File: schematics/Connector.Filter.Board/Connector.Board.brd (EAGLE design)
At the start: 159.4 x 72.1 mm, 95 parts, among them U1 AD8244, U2 AD8244, U3 AD8244, U4 AD8244, U5 AD8244, U6 AD8244, U7 AD8244, U8 AD8244, U9 AD8244, X1 EEGCON, X2 EITCON

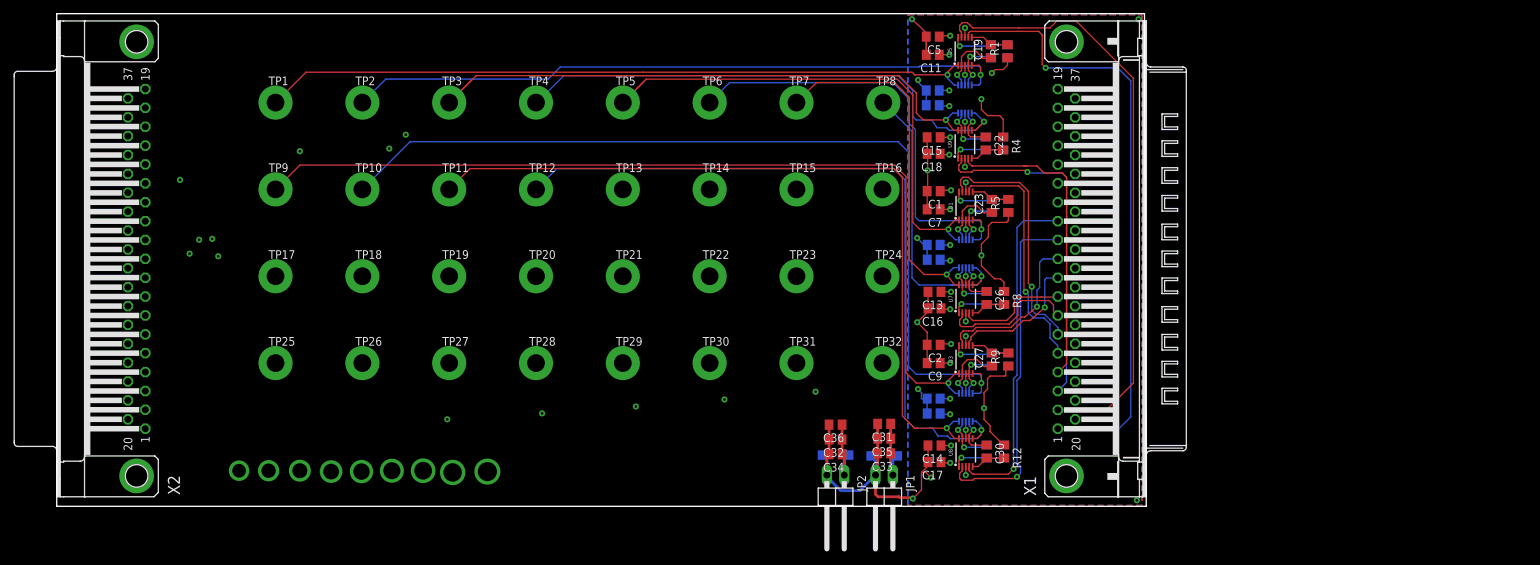
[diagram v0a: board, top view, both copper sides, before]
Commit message: Renaming Sch and Brd but not matching yet
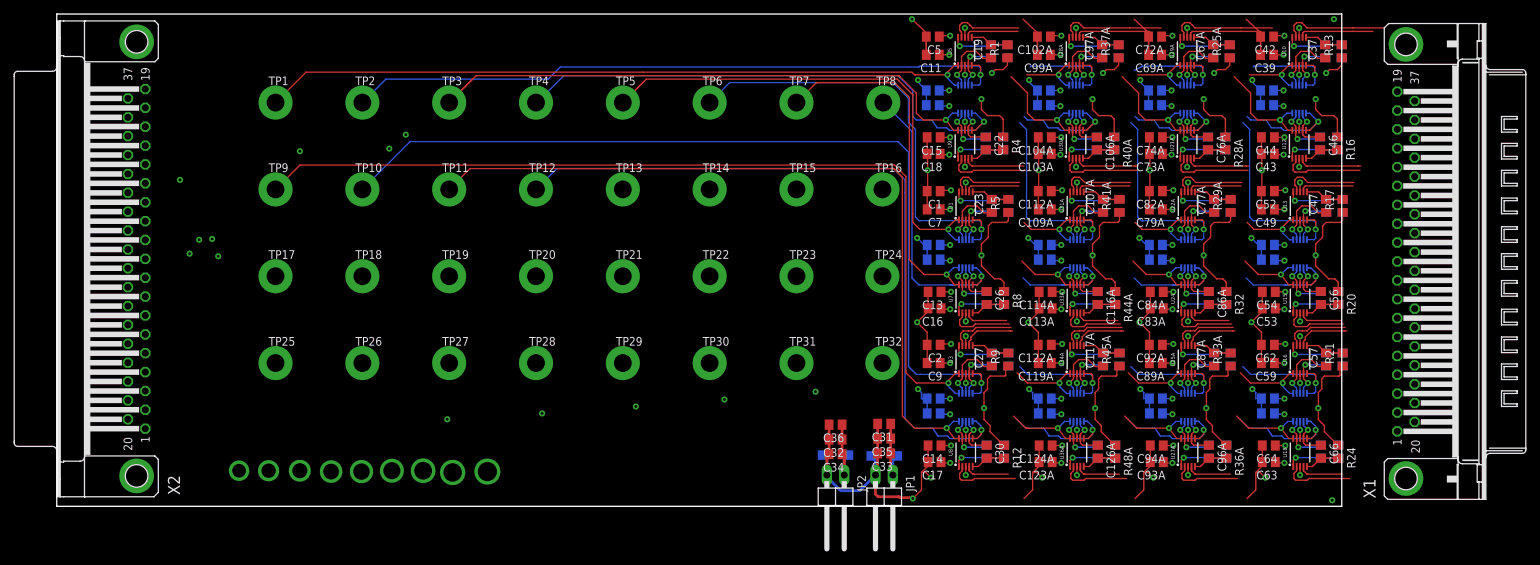
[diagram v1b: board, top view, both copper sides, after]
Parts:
- added C100A, C101A, C102A, C103A, C104A, C105A, C109A, C110A, C111A, C112A, C113A, C114A, C119A, C120A, C121A, C122A, C123A, C124A, C39, C40, C41, C42, C43, C44, C45, C49, C50, C51, C52, C53, C54, C59, C60, C61, C62, C63, C64, C69A, C70A, C71A, C72A, C73A, C74A, C75A, C79A, C80A, C81A, C82A, C83A, C84A, C89A, C90A, C91A, C92A, C93A, C94A, C99A: 0.1uF, resistor:C0805
- added C106A, C107A, C108A, C115A, C116A, C117A, C118A, C125, C126A, C37, C38, C46, C47, C48, C55, C56, C57, C58, C65, C66, C67A, C68A, C76A, C77A, C78A, C85A, C86A, C87A, C88A, C95A, C96A, C97A, C98A: (no value), resistor:C0805
- added R13, R14, R15, R16, R17, R18, R19, R20, R21, R22, R23, R24, R25A, R26A, R27A, R28A, R29A, R30A, R31, R32, R33A, R34A, R35A, R36A, R37A, R38A, R39A, R40A, R41A, R42A, R43A, R44A, R45A, R46A, R47, R48A: (no value), resistor:R0805
- added U10, U11, U12, U13, U14, U15, U16, U17, U18, U19A, U20A, U21A, U22A, U23A, U24, U25A, U26A, U27A, U28A, U29A, U30A, U31A, U32A, U33A, U34A, U35A, U36A: AD8244, AD8244:MSOP10
- moved X1 49.7 mm to (198.2, 55.2)
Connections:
- new net BUF13: C37.1, C97A.1, U10.2, U11.2, U28A.2, U29A.2
- new net BUF14: C38.1, C98A.1, U10.4, U11.4, U28A.4, U29A.4
- new net BUF15: C105A.1, C45.1, U11.9, U12.9, U29A.9, U30A.9
- new net BUF16: C106A.1, C46.1, U11.7, U12.7, U29A.7, U30A.7
- new net BUF17: C107A.1, C47.1, U13.2, U14.2, U31A.2, U32A.2
- new net BUF18: C108A.1, C48.1, U13.4, U14.4, U31A.4, U32A.4
- new net BUF19: C115A.1, C55.1, U14.9, U15.9, U32A.9, U33A.9
- new net BUF20: C116A.1, C56.1, U14.7, U15.7, U32A.7, U33A.7
- new net BUF21: C117A.1, C57.1, U16.2, U17.2, U34A.2, U35A.2
- new net BUF22: C118A.1, C58.1, U16.4, U17.4, U34A.4, U35A.4
- new net BUF23: C125.1, C65.1, U17.9, U18.9, U35A.9, U36A.9
- new net BUF24: C126A.1, C66.1, U17.7, U18.7, U35A.7, U36A.7
- new net BUF25: C67A.1, U19A.2, U20A.2
- new net BUF26: C68A.1, U19A.4, U20A.4
- new net BUF27: C75A.1, U20A.9, U21A.9
- new net BUF28: C76A.1, U20A.7, U21A.7
- new net BUF29: C77A.1, U22A.2, U23A.2
- new net BUF30: C78A.1, U22A.4, U23A.4
- new net BUF31: C85A.1, U23A.9, U24.9
- new net BUF32: C86A.1, U23A.7, U24.7
- new net BUF33: C87A.1, U25A.2, U26A.2
- new net BUF34: C88A.1, U25A.4, U26A.4
- new net BUF35: C95A.1, U26A.9, U27A.9
- new net BUF36: C96A.1, U26A.7, U27A.7
- new net FILT10_BUF1: U16.9
- new net FILT10_BUF2: U25A.9
- new net FILT10_OUT1: C58.2, R22.2, U16.10
- new net FILT10_OUT2: C88A.2, R34A.2, U25A.10
- new net FILT11_BUF1: U18.2
- new net FILT11_BUF2: U27A.2
- new net FILT11_OUT1: C65.2, R23.2, U18.1
- new net FILT11_OUT2: C95A.2, R35A.2, U27A.1
- new net FILT12_BUF1: U18.4
- new net FILT12_BUF2: U27A.4
- new net FILT12_OUT1: C66.2, R24.2, U18.5
- new net FILT12_OUT2: C96A.2, R36A.2, U27A.5
- new net FILT14_OUT: C98A.2, R38A.2, U28A.10
- new net FILT15_OUT: C105A.2, R39A.2, U30A.1
- new net FILT16_OUT: C106A.2, R40A.2, U30A.5
- new net FILT17_OUT: C107A.2, R41A.2, U31A.6
- new net FILT18_OUT: C108A.2, R42A.2, U31A.10
- new net FILT19_OUT: C115A.2, R43A.2, U33A.1
- new net FILT1_BUF1: U10.7
- new net FILT1_OUT1: C37.2, R13.2, U10.6
- new net FILT20_OUT: C116A.2, R44A.2, U33A.5
- new net FILT21_OUT: C117A.2, R45A.2, U34A.6
- new net FILT22_OUT: C118A.2, R46A.2, U34A.10
- new net FILT23_OUT: C125.2, R47.2, U36A.1
- new net FILT24_OUT: C126A.2, R48A.2, U36A.5
- new net FILT25_OUT: C67A.2, R25A.2, U19A.6
- new net FILT26_OUT: C68A.2, R26A.2, U19A.10
- new net FILT27_OUT: C75A.2, R27A.2, U21A.1
- new net FILT28_OUT: C76A.2, R28A.2, U21A.5
- new net FILT2_BUF1: U10.9
- new net FILT2_OUT1: C38.2, R14.2, U10.10
- new net FILT31_OUT: C85A.2, R31.2, U24.1
- new net FILT32_OUT: C86A.2, R32.2, U24.5
- new net FILT3_BUF1: U12.2
- new net FILT3_OUT1: C45.2, R15.2, U12.1
- new net FILT4_BUF1: U12.4
- new net FILT4_OUT1: C46.2, R16.2, U12.5
- new net FILT5_BUF1: U13.7
- new net FILT5_BUF2: U22A.7
- new net FILT5_OUT1: C47.2, R17.2, U13.6
- new net FILT5_OUT2: C77A.2, R29A.2, U22A.6
- new net FILT6_BUF1: U13.9
- new net FILT6_BUF2: U22A.9
- new net FILT6_OUT1: C48.2, R18.2, U13.10
- new net FILT6_OUT2: C78A.2, R30A.2, U22A.10
- new net FILT7_BUF1: U15.2
- new net FILT7_OUT1: C55.2, R19.2, U15.1
- new net FILT8_BUF1: U15.4
- new net FILT8_OUT1: C56.2, R20.2, U15.5
- new net FILT9_BUF1: U16.7
- new net FILT9_BUF2: U25A.7
- new net FILT9_OUT1: C57.2, R21.2, U16.6
- new net FILT9_OUT2: C87A.2, R33A.2, U25A.6
- new net PIN33: U10.1, U11.1
- new net PIN34: U10.5, U11.5
- new net PIN35: U11.10, U12.10
- new net PIN36: U11.6, U12.6
- new net PIN37: U13.1, U14.1
- new net PIN38: U13.5, U14.5
- new net PIN39: U14.10, U15.10
- new net PIN40: U14.6, U15.6
- new net PIN41: U16.1, U17.1
- new net PIN42: U16.5, U17.5
- new net PIN43: U17.10, U18.10
- new net PIN44: U17.6, U18.6
- new net PIN53: U25A.1, U26A.1
- new net PIN54: U25A.5, U26A.5
- new net PIN55: U26A.10, U27A.10
- new net PIN56: U26A.6, U27A.6
- net FILT13_BUF: now also U28A.7
- net FILT14_BUF: now also U28A.9
- net FILT15_BUF: now also U30A.2
- net FILT16_BUF: now also U30A.4
- net FILT17_BUF: now also U31A.7
- net FILT18_BUF: now also U31A.9
- net FILT19_BUF: now also U33A.2
- net FILT20_BUF: now also U33A.4
- net FILT21_BUF: now also U34A.7
- net FILT22_BUF: now also U34A.9
- net FILT23_BUF: now also U36A.2
- net FILT24_BUF: now also U36A.4
- net FILT25_BUF: now also U19A.7
- net FILT26_BUF: now also U19A.9
- net FILT27_BUF: now also U21A.2
- net FILT28_BUF: now also U21A.4
- net FILT31_BUF: now also U24.2
- net FILT32_BUF: now also U24.4
- net FILT3_OUT: now also C97A.2, R37A.2, U28A.6
- net GND: now also C100A.2, C101A.2, C102A.2, C103A.2, C104A.2, C109A.2, C110A.2, C111A.2, C112A.2, C113A.2, C114A.2, C119A.2, C120A.2, C121A.2, C122A.2, C123A.2, C124A.2, C39.2, C40.2, C41.2, C42.2, C43.2, C44.2, C49.2, C50.2, C51.2, C52.2, C53.2, C54.2, C59.2, C60.2, C61.2, C62.2, C63.2, C64.2, C69A.2, C70A.2, C71A.2, C72A.2, C73A.2, C74A.2, C79A.2, C80A.2, C81A.2, C82A.2, C83A.2, C84A.2, C89A.2, C90A.2, C91A.2, C92A.2, C93A.2, C94A.2, C99A.2, R13.1, R14.1, R15.1, R16.1, R17.1, R18.1, R19.1, R20.1, R21.1, R22.1, R23.1, R24.1, R25A.1, R26A.1, R27A.1, R28A.1, R29A.1, R30A.1, R31.1, R32.1, R33A.1, R34A.1, R35A.1, R36A.1, R37A.1, R38A.1, R39A.1, R40A.1, R41A.1, R42A.1, R43A.1, R44A.1, R45A.1, R46A.1, R47.1, R48A.1
- net PIN13: now also U28A.1, U29A.1
- net PIN14: now also U28A.5, U29A.5
- net PIN15: now also U29A.10, U30A.10
- net PIN16: now also U29A.6, U30A.6
- net PIN17: now also U31A.1, U32A.1
- net PIN18: now also U31A.5, U32A.5
- net PIN19: now also U32A.10, U33A.10
- net PIN20: now also U32A.6, U33A.6
- net PIN21: now also U34A.1, U35A.1
- net PIN22: now also U34A.5, U35A.5
- net PIN23: now also U35A.10, U36A.10
- net PIN24: now also U35A.6, U36A.6
- net PIN25: now also U19A.1, U20A.1
- net PIN26: now also U19A.5, U20A.5
- net PIN27: now also U20A.10, U21A.10
- net PIN28: now also U20A.6, U21A.6
- net PIN29: now also U22A.1, U23A.1
- net PIN30: now also U22A.5, U23A.5
- net PIN31: now also U23A.10, U24.10
- net PIN32: now also U23A.6, U24.6
- net V+: now also C100A.1, C103A.1, C109A.1, C110A.1, C113A.1, C119A.1, C120A.1, C123A.1, C39.1, C40.1, C43.1, C49.1, C50.1, C53.1, C59.1, C60.1, C63.1, C69A.1, C70A.1, C73A.1, C79A.1, C80A.1, C83A.1, C89A.1, C90A.1, C93A.1, C99A.1, U10.3, U11.3, U12.3, U13.3, U14.3, U15.3, U16.3, U17.3, U18.3, U19A.3, U20A.3, U21A.3, U22A.3, U23A.3, U24.3, U25A.3, U26A.3, U27A.3, U28A.3, U29A.3, U30A.3, U31A.3, U32A.3, U33A.3, U34A.3, U35A.3, U36A.3
- net V-: now also C101A.1, C102A.1, C104A.1, C111A.1, C112A.1, C114A.1, C121A.1, C122A.1, C124A.1, C41.1, C42.1, C44.1, C51.1, C52.1, C54.1, C61.1, C62.1, C64.1, C71A.1, C72A.1, C74A.1, C81A.1, C82A.1, C84A.1, C91A.1, C92A.1, C94A.1, U10.8, U11.8, U12.8, U13.8, U14.8, U15.8, U16.8, U17.8, U18.8, U19A.8, U20A.8, U21A.8, U22A.8, U23A.8, U24.8, U25A.8, U26A.8, U27A.8, U28A.8, U29A.8, U30A.8, U31A.8, U32A.8, U33A.8, U34A.8, U35A.8, U36A.8
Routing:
- net GND: track 310.2 -> 875.9 mm, vias 14 -> 44
- net V+: track 165.1 -> 621.4 mm, vias 15 -> 60
- net V-: track 178.3 -> 470.2 mm, vias 15 -> 60
- net FILT1_BUF: track 90.6 -> 7.96 mm, vias 1 -> 0
- net FILT2_BUF: track 88.9 -> 11.0 mm
- net FILT12_BUF: track 49.6 -> 6.55 mm, vias 1 -> 0
- net FILT11_BUF: track 51.2 -> 10.3 mm, vias 1 -> 0
- net FILT3_BUF: track 50.1 -> 11.9 mm, vias 1 -> 0
- net FILT4_BUF: track 45.3 -> 8.96 mm
- net PIN30: track 97.5 -> 127.9 mm, vias 0 -> 1
- net PIN18: track 58.5 -> 88.9 mm, vias 1 -> 2
- net PIN38: track 0.00 -> 30.4 mm, vias 0 -> 1
- net FILT5_BUF: track 35.8 -> 7.96 mm, vias 1 -> 0
- net FILT6_BUF: track 36.3 -> 11.0 mm, vias 1 -> 0
- net BUF13: track 0.00 -> 20.3 mm, vias 0 -> 2
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- removed copper zone on layer 1, net GND
- removed copper zone on layer 16, net GND
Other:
- board size 159.4 x 72.1 mm -> 188 x 72 mm
